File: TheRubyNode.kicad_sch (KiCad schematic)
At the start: 65 parts, among them J1 USB4085-GF-A_REVB, J2 Conn_02x01, J3 Conn_02x01, J4 Conn_01x02, J5 91930-21111LF, J6 Conn_01x04, J7 Conn_01x03, Q1 Si2307, SW1 SW_SPST, SW2 SW_Push, SW3 SW_Push, SW4 SW_Push, U1 INA219AxD, U2 LoRa1121F33-2G4, U3 SC189Z, U4 MCP73833-AMI-UN, U5 ESP32-S3-WROOM-1, U6 USBLC6-2SC6, U7 ISL97519A

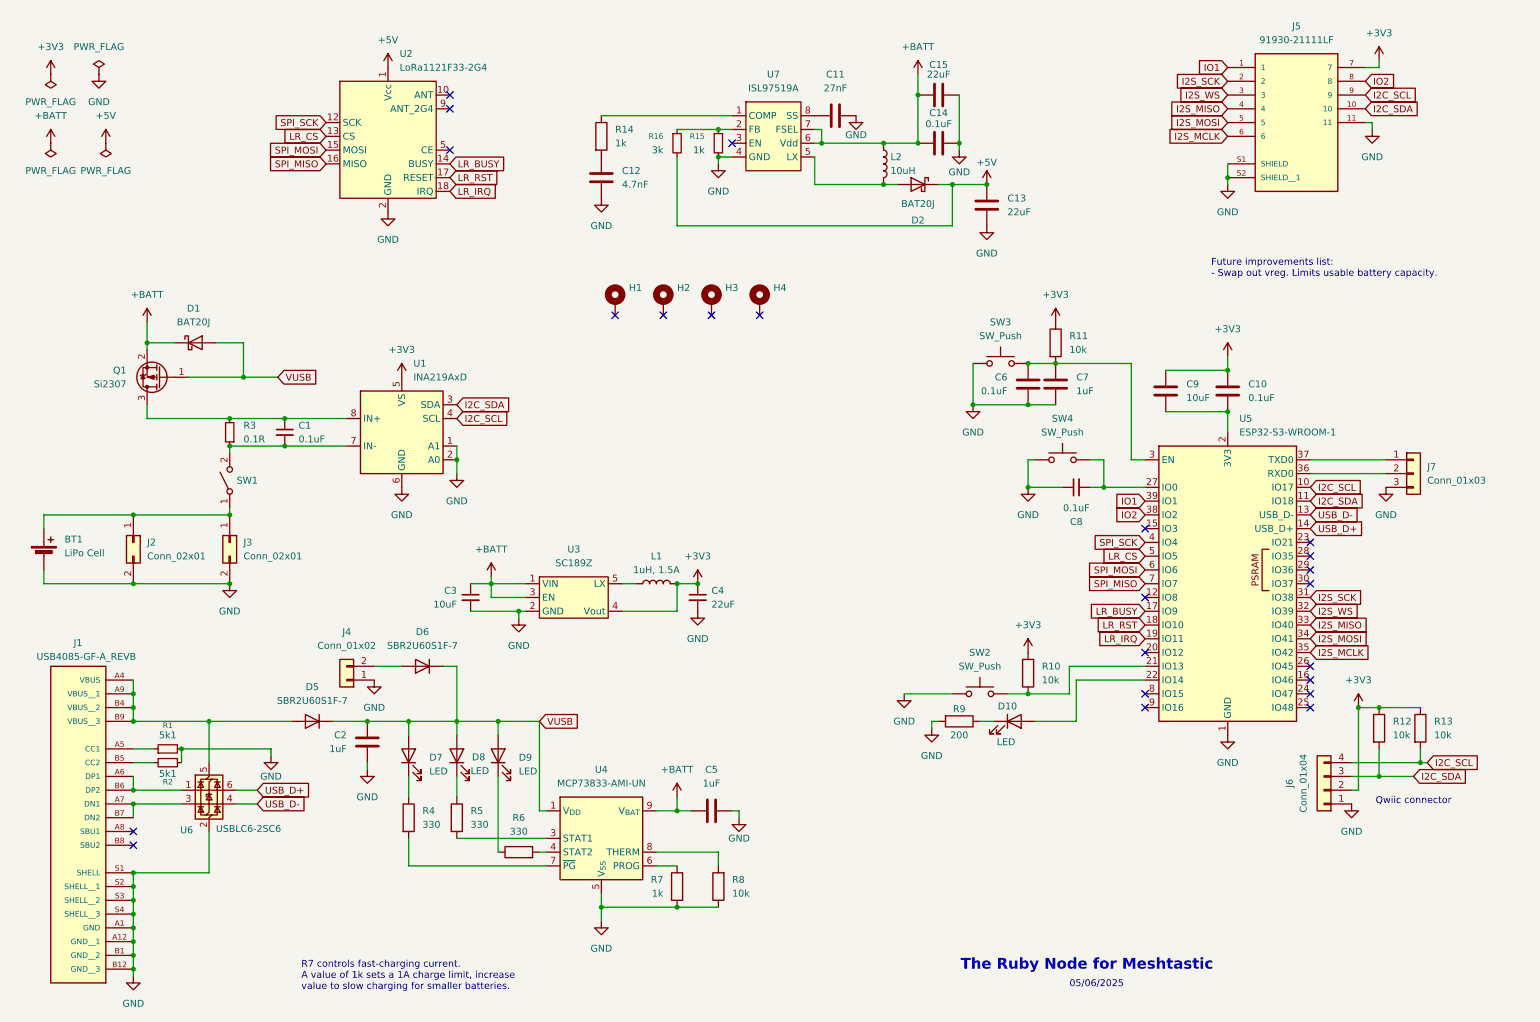
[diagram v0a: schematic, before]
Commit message: Add PCB design
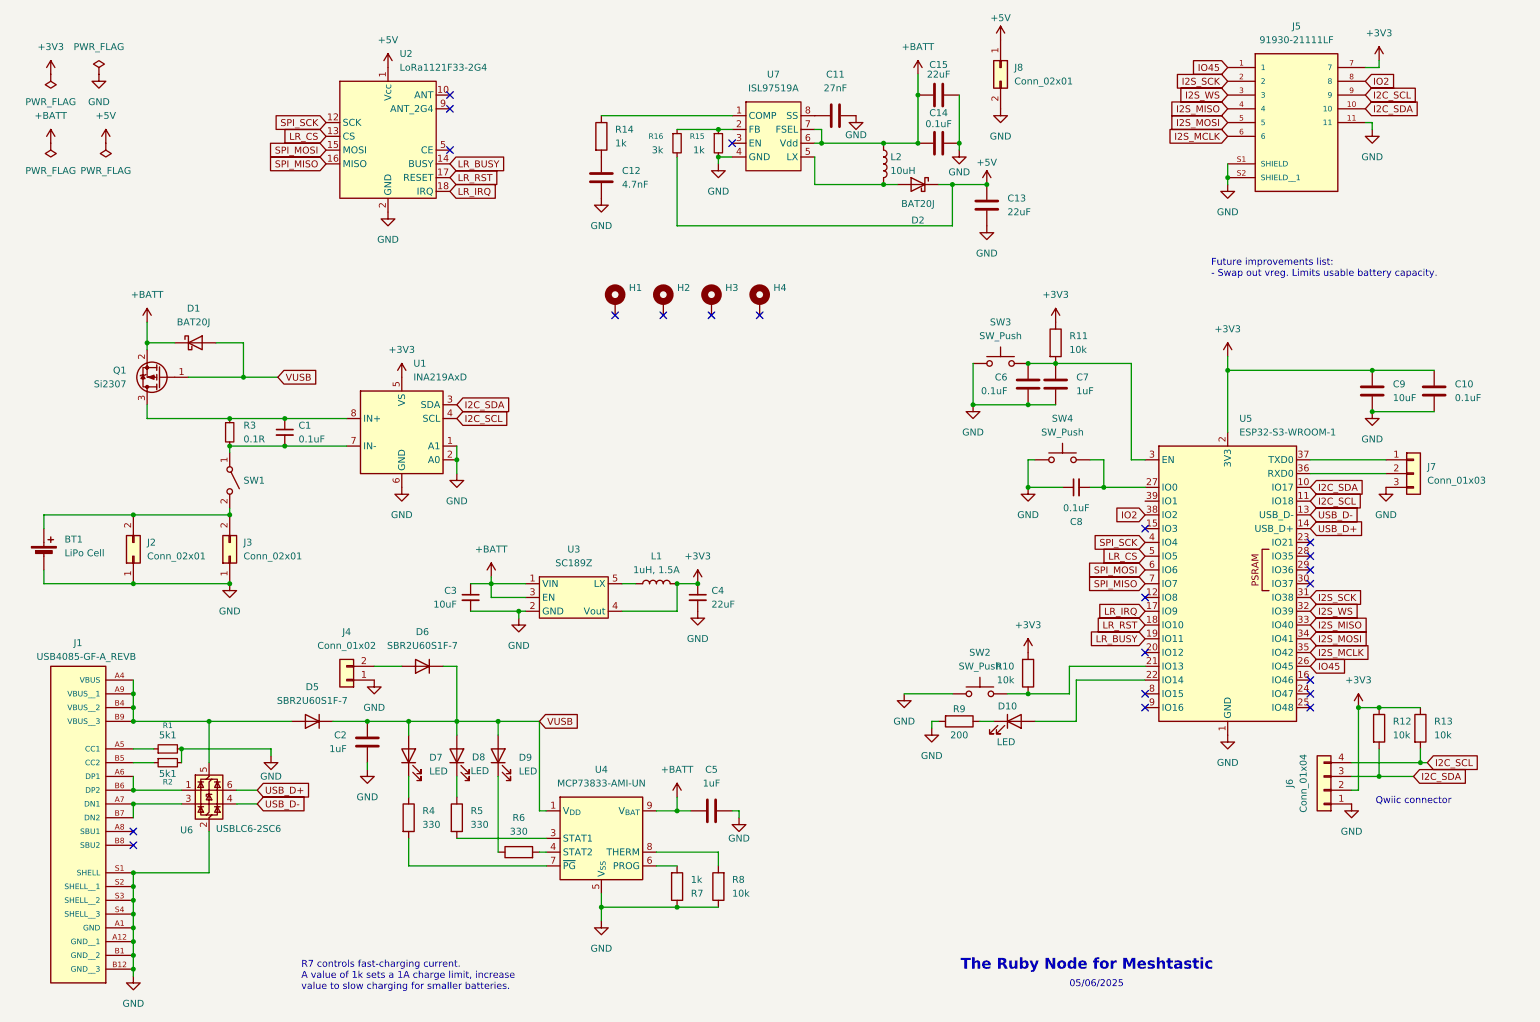
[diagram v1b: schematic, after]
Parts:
- added J8: Conn_02x01, Connector_JST:JST_PH_B2B-PH-SM4-TB_1x02-1MP_P2.00mm_Vertical, symbol Connector_Generic:Conn_02x01
- SW2: footprint Connector_JST:JST_PH_S2B-PH-SM4-TB_1x02-1MP_P2.00mm_Horizontal -> Connector_JST:JST_PH_B2B-PH-SM4-TB_1x02-1MP_P2.00mm_Vertical
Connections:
- net +3V3: now also U5.2 (3V3)
- net +5V: now also J8.1 (Pin_1)
- net GND: now also C10.2, C9.2, J2.1 (Pin_1), J3.1 (Pin_1), R2.2, R7.1, J8.2 (Pin_2); no longer J2.2 (Pin_2), J3.2 (Pin_2), R2.1, R7.2
- net I2C_SCL: now also U5.11 (IO18); no longer U5.10 (IO17)
- net I2C_SDA: now also U5.10 (IO17); no longer U5.11 (IO18)
- net LR_BUSY: now also U5.19 (IO11); no longer U5.17 (IO9)
- net LR_IRQ: now also U5.17 (IO9); no longer U5.19 (IO11)
- net at C1.1, Q1.3 (D), U1.8 (IN+): now also R3.1; no longer R3.2
- net at C1.2, U1.7 (IN-): now also R3.2, SW1.1 (A); no longer R3.1, SW1.2 (B)
- net at U4.6 (PROG): now also R7.2; no longer R7.1
- net IO45: now reaches U5.26 (IO45)
- net IO45: now also J5.1
- net at J1.B5 (CC2): now also R2.1; no longer R2.2
- net IO1: no longer names the net of U5.39 (IO1)
- net IO1: no longer J5.1
- new net: BT1.1 (+), J2.2 (Pin_2), J3.2 (Pin_2), SW1.2 (B)
- no-connect marks 23 -> 22
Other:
- moved on the sheet: C10, C9, J2, J3, R10, R2, R3, SW1

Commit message: Finalise rev 1.0 of PCB
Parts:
- J6: footprint Connector_JST:JST_SH_SM04B-SRSS-TB_1x04-1MP_P1.00mm_Horizontal -> Connector_JST:JST_SH_BM04B-SRSS-TB_1x04-1MP_P1.00mm_Vertical
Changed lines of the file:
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@@
 			)
 		)
-		(property "Footprint" "Connector_JST:JST_SH_SM04B-SRSS-TB_1x04-1MP_P1.00mm_Horizontal"
+		(property "Footprint" "Connector_JST:JST_SH_BM04B-SRSS-TB_1x04-1MP_P1.00mm_Vertical"
 			(at 254 157.48 0)
 			(effects
